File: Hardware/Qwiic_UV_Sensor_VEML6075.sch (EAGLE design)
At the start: 27 parts, among them J1 GATORGATOR_MINI, J2 GATORGATOR_MINI, J3 GATORGATOR_MINI, J4 GATORGATOR_MINI, J5 GATORGATOR_MINI, J6 GATORGATOR_MINI, J7 GATORGATOR_MINI, J8 GATORGATOR_MINI, U1 VEML6075

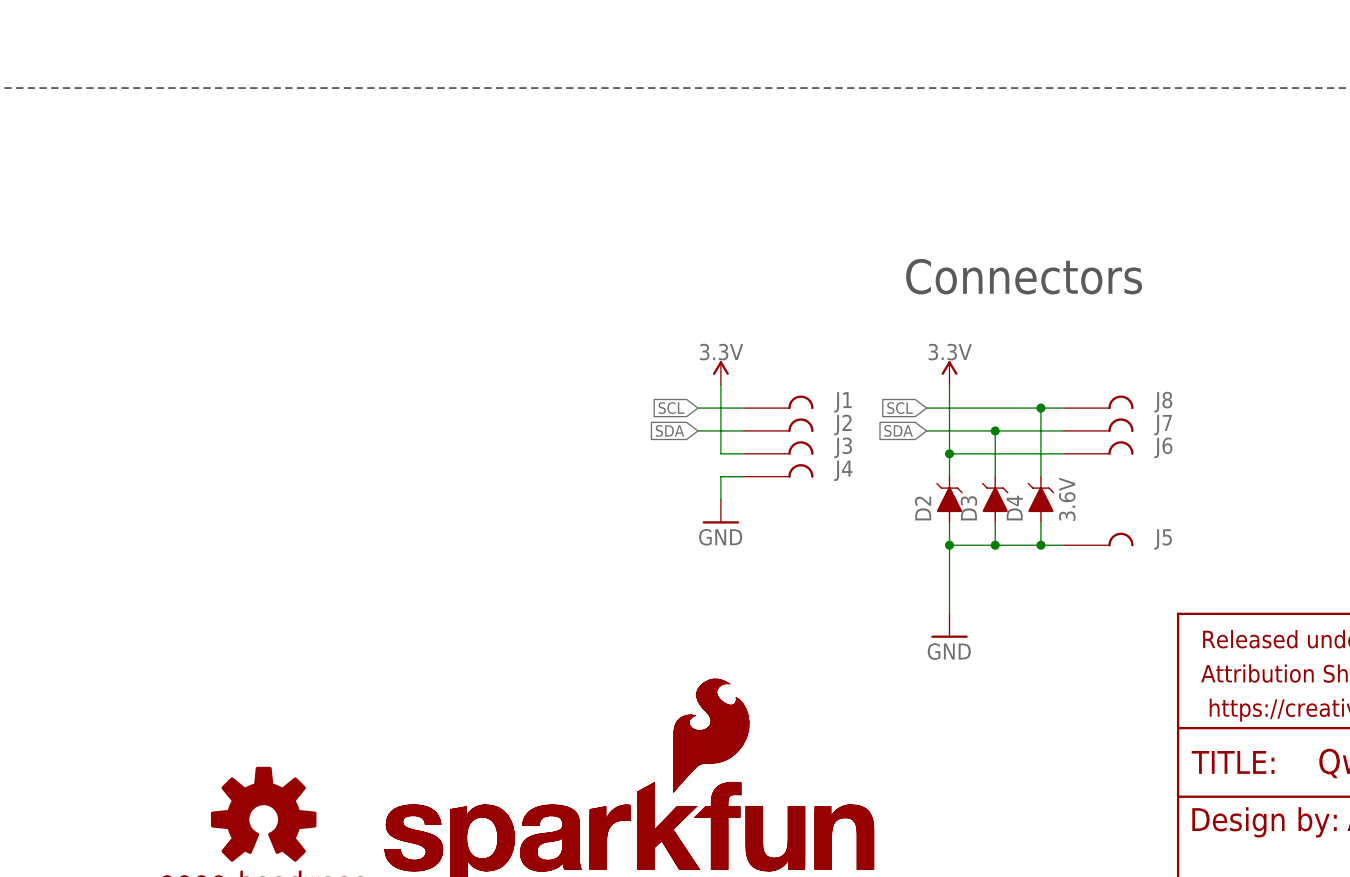
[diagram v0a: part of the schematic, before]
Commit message: post checklist changes
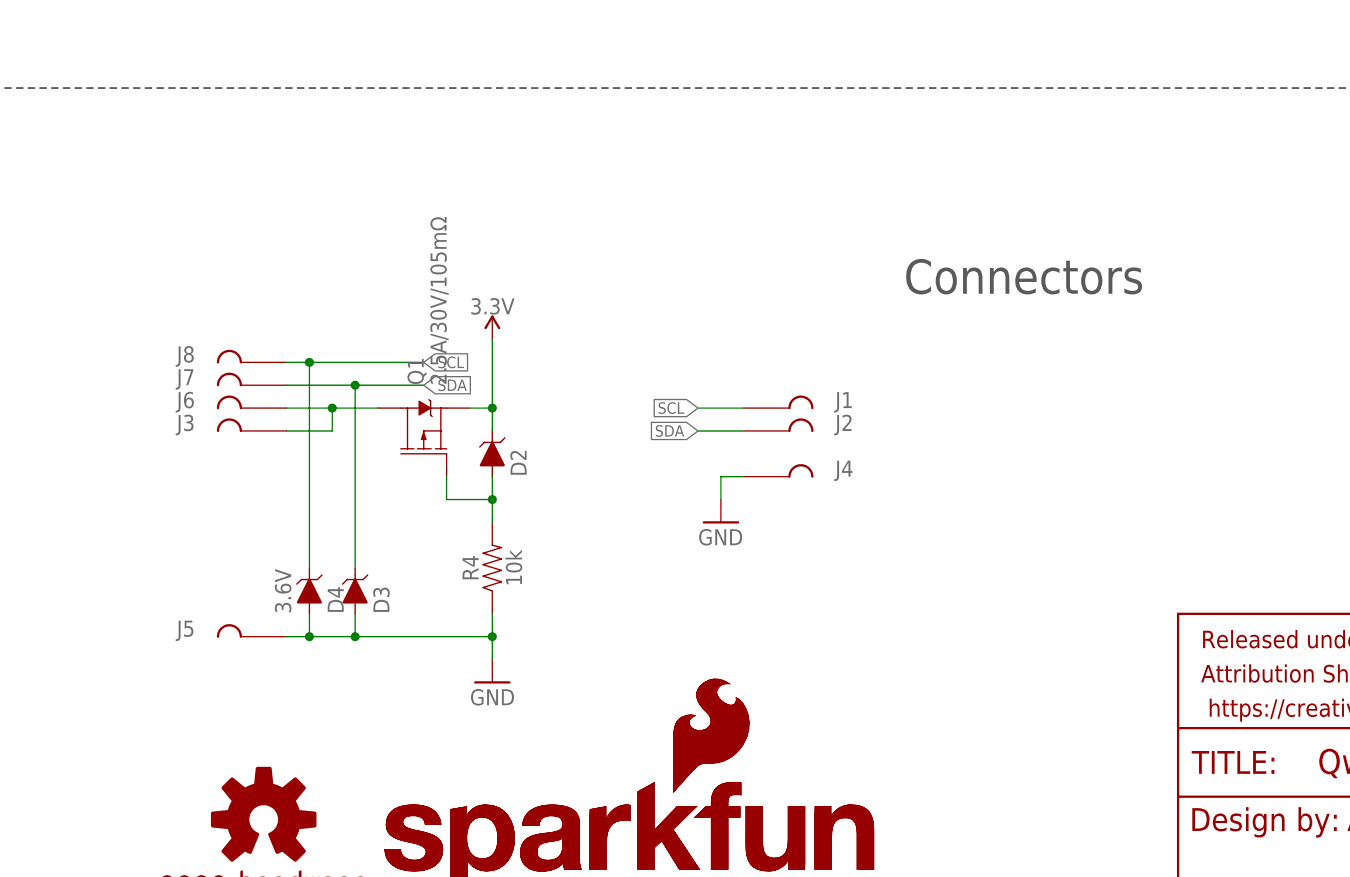
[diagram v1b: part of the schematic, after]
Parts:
- added Q1: 2.5A/30V/105mΩ, SparkFun-DiscreteSemi:MOSFET_PCH-DMG2307L
- added R4: 10k, SparkFun-Resistors:10KOHM-0603-1/10W-1%
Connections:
- new net N$1: J3.P$1, J6.P$1, Q1.D
- new net N$4: D2.A, Q1.G, R4.2
- net 3.3V: now also Q1.S; no longer J3.P$1, J6.P$1
- net GND: now also R4.1; no longer D2.A
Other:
- moved on the sheet: D2, D3, D4, J3, J5, J6, J7, J8
